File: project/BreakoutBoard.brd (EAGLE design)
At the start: 45.2 x 45.2 mm, 2 parts, among them J1 XF2L-2435-1, X1 LCD

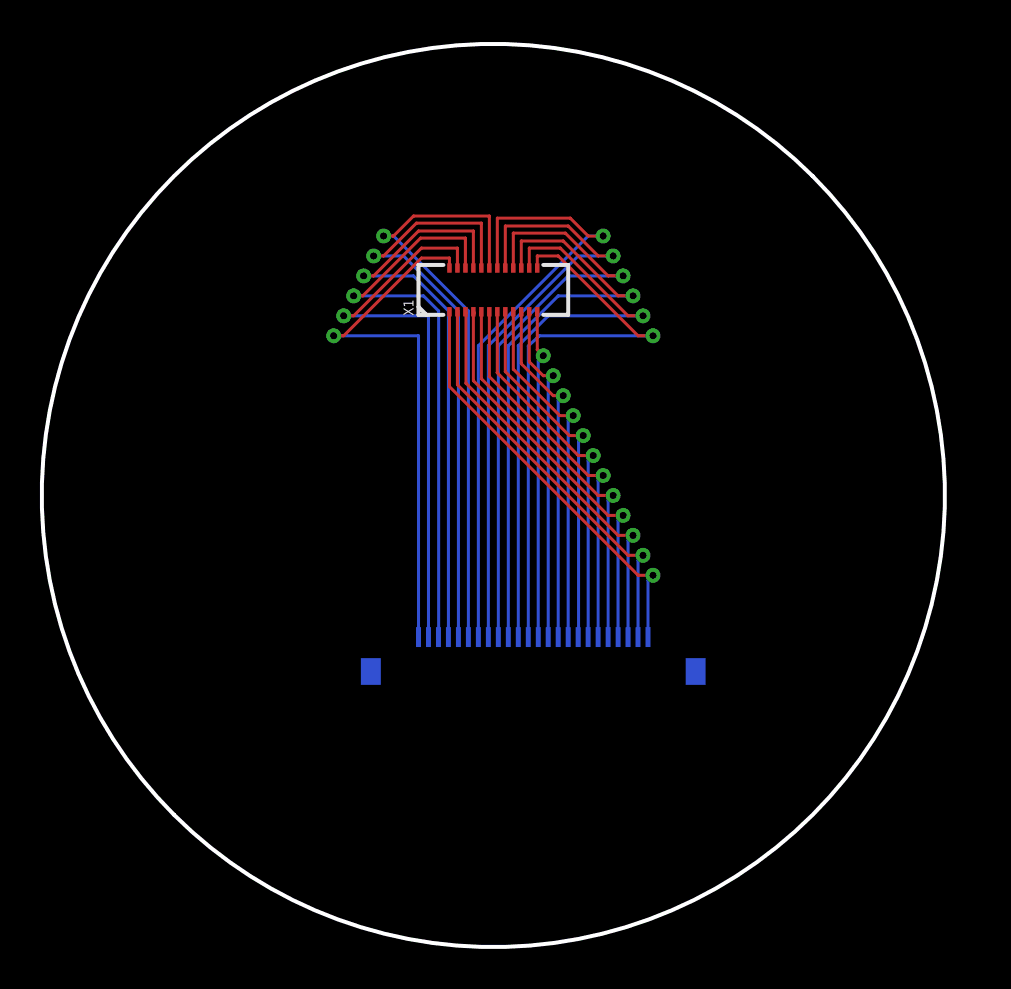
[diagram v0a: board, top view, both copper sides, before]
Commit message: Layout complete
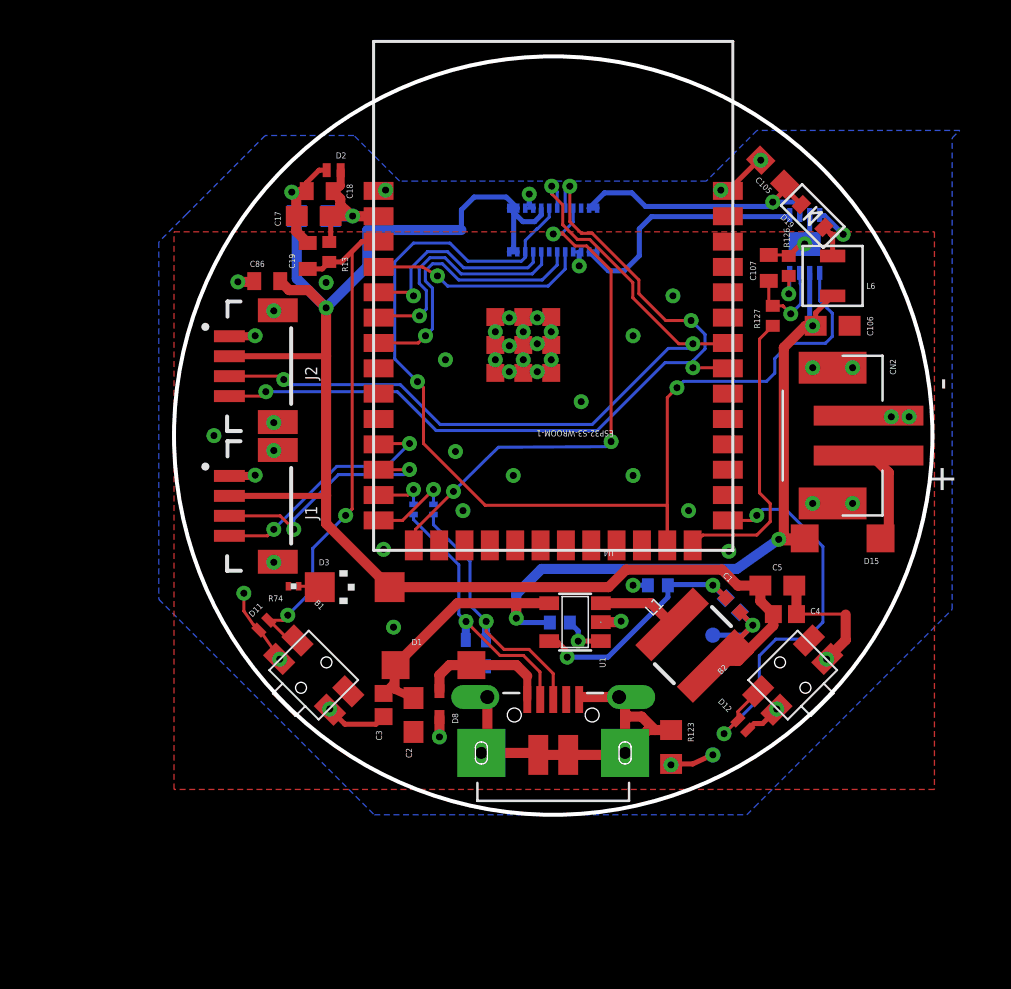
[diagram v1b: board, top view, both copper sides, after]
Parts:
- added B1: RESET, alps:SKSCLDE010
- added B2: BOOT, alps:SKSCLDE010
- added C1: 22pF/50V, SparkFun-Capacitors:0402-TIGHT
- added C105: 2.2uF/16V, rcl:C0603
- added C106: 4.7uF/16V, rcl:C0603
- added C107: 22pF/50V, rcl:C0402
- added C17: 10uF/16V, rcl:C0603
- added C18: 0.1uF/10V, rcl:C0402
- added C19: 1uF/16V, rcl:C0402
- added C2, C5: 10uF/16V, SparkFun-Capacitors:0603
- added C3, C4: 0.1uF/10V, SparkFun-Capacitors:0402
- added C86: (no value), rcl:C0402
- added CN2: (no value), adafruit:JST-PH-2-SMT
- added D1, D15: (no value), diode:SOD123
- added D10, D8, D9: LESD5D5.0CT1G, discrete:SOD523
- added D11, D12, D2: LESD8D3.3CAT5G, discrete:SOD882
- added D19: (no value), adafruit:SOD-523
- added D3: (no value), led:CHIPLED_1206
- added J2: I2C2, SparkFun-Connectors:JST04_1MM_VERT
- added J3: LCD, ER-CON0.4-24P:OK-24F024-04
- added L1: 2.2μH, SparkFun-Coils:INDUCTOR_4X4MM
- added L6: 10uH_0.8A, discrete:L3012S
- added R1, R13: 10K, rcl:R0402
- added R111, R112: 0, rcl:R0201
- added R12, R123: 0, rcl:R0603
- added R126: 6.6, rcl:R0402
- added R127: 10, rcl:R0402
- added R2: 680K, rcl:R0402
- added R3: 150K, rcl:R0402
- added R74: 51, rcl:R0201
- added TP1, TP2: (no value), SparkFun-Connectors:PAD.03X.03
- added U1: SY8088, discrete:SOT23-5
- added U15: BD60A60NUX, discrete:VSON008X2030
- added U4: ESP32-S3-WROOM-1, espressif:QFN60_ESP32-S3-WROOM-1_EXP
- J1: value XF2L-2435-1 -> I2C1; device con-omron:XF2L-2435-1 -> SparkFun-Connectors:JST04_1MM_VERT
- X1: value LCD -> (none); device ER-CON0.4-24P:OK-24F024-04 -> Adafruit ItsyBitsy nRF52840 Express:MICROBUILDER_4UCONN_20329
- moved X1 21.5 mm to (19.0, 5.00), turned to 0 degrees
- moved J1 18.1 mm to (2.00, 15.5), flipped to the top, turned to 270 degrees
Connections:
- removed net N$10: J1.10, X1.10
- removed net N$11: J1.11, X1.11
- removed net N$12: J1.12, X1.12
- removed net N$13: J1.13, X1.13
- removed net N$14: J1.14, X1.14
- removed net N$15: J1.15, X1.15
- removed net N$16: J1.16, X1.16
- removed net N$17: J1.17, X1.17
- removed net N$18: J1.18, X1.18
- removed net N$19: J1.19, X1.19
- removed net N$20: J1.20, X1.20
- removed net N$21: J1.21, X1.21
- removed net N$22: J1.22, X1.22
- removed net N$23: J1.23, X1.23
- removed net N$24: J1.24, X1.24
- removed net N$3: J1.3, X1.3
- removed net N$5: J1.5, X1.5
- new net ESP_3V3: C17.1, C18.1, D2.C, R12.2, R13.1, U4.2
- new net GND: B1.1, B2.1, C105.2, C106.2, C107.2, C17.2, C18.2, C19.2, C2.2, C3.2, C4.2, C5.2, C86.2, CN2.2, D10.A, D11.A, D12.A, D2.A, D8.A, D9.A, J1.1, J2.1, J3.15, J3.16, J3.3, J3.4, R123.1, R126.1, R3.1, R74.1, TP2.1, U1.2, U15.7, U15.PAD, U4.1, U4.40, U4.41, U4.42, U4.43, U4.44, U4.45, U4.46, U4.47, U4.48, U4.49
- new net GPIO0: B2.3, D12.C, U4.27
- new net GPIO18: J1.4, U4.11
- new net GPIO19: R111.2, U4.13
- new net GPIO20: R112.2, U4.14
- new net GPIO3: J3.21, U4.15
- new net GPIO4: J3.5, U4.4
- new net GPIO40: J2.4, J3.20, U4.33
- new net GPIO41: J2.3, J3.19, U4.34
- new net GPIO45: R127.1, U4.26
- new net GPIO48: J3.10, J3.18, U15.1, U4.25
- new net GPIO5: J3.9, U4.5
- new net GPIO6: J3.8, U4.6
- new net GPIO7: J3.6, U4.7
- new net GPIO8: J1.3, U4.12
- new net LED_A: C105.1, D19.K, J3.23, J3.24, U15.6
- new net LED_DIM: C107.1, R127.2, U15.3
- new net LED_K: J3.1, J3.2, U15.5
- new net MCU_RST: B1.3, C19.1, D11.C, R13.2, U4.3
- new net MCU_VDD: C1.1, C4.1, C5.1, C86.1, D3.A, J1.2, J2.2, J3.11, J3.12, J3.13, J3.14, J3.17, L1.P$2, R12.1, R2.2, TP1.1
- new net USB_5V: C106.1, C2.1, C3.1, D1.C, D15.C, L6.P$1, R1.1, U1.4, U15.2
- new net USB_DN: D9.C, R111.1, X1.D-
- new net USB_DP: D10.C, R112.1, X1.D+
- new net USB_G: R123.2, X1.BASE@1, X1.BASE@2, X1.GND, X1.SPRT@1, X1.SPRT@2, X1.SPRT@3, X1.SPRT@4
- new net USB_VBUS: D1.A, D8.C, X1.VBUS
- net N$1: now also D19.A, L6.P$2, U15.8; no longer J1.1, X1.1
- net N$2: now also D3.C, R74.2; no longer J1.2, X1.2
- net N$4: now also CN2.1, D15.A; no longer J1.4, X1.4
- net N$6: now also R1.2, U1.1; no longer J1.6, X1.6
- net N$7: now also L1.P$1, U1.3; no longer J1.7, X1.7
- net N$8: now also C1.2, R2.1, R3.2, U1.5; no longer J1.8, X1.8
- net N$9: now also R126.2, U15.4; no longer J1.9, X1.9
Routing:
- net MCU_VDD: track 0.00 -> 84.3 mm, vias 0 -> 2
- net GPIO48: track 0.00 -> 56.4 mm, vias 0 -> 2
- net USB_5V: track 0.00 -> 48.7 mm, vias 0 -> 3
- net GPIO40: track 0.00 -> 41.8 mm, vias 0 -> 4
- net GPIO41: track 0.00 -> 40.5 mm, vias 0 -> 3
- net GND: track 0.00 -> 37.8 mm, vias 0 -> 56
- net N$18: track 31.3 -> 0.00 mm, vias 1 -> 0
- net N$17: track 30.8 -> 0.00 mm, vias 1 -> 0
- net N$19: track 30.5 -> 0.00 mm, vias 1 -> 0
- net N$16: track 30.4 -> 0.00 mm, vias 1 -> 0
- net N$20: track 30.1 -> 0.00 mm, vias 1 -> 0
- net N$15: track 30.0 -> 0.00 mm, vias 1 -> 0
- net N$21: track 29.6 -> 0.00 mm, vias 1 -> 0
- net N$14: track 29.6 -> 0.00 mm, vias 1 -> 0
- net N$22: track 29.2 -> 0.00 mm, vias 1 -> 0
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- added copper zone on layer 1, net GND
- added copper zone on layer 16, net GND
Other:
- board size 45.2 x 45.2 mm -> 38 x 38 mm
